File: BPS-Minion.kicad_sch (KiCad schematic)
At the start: 11 parts, among them U12 MIC5317-2.5xM5

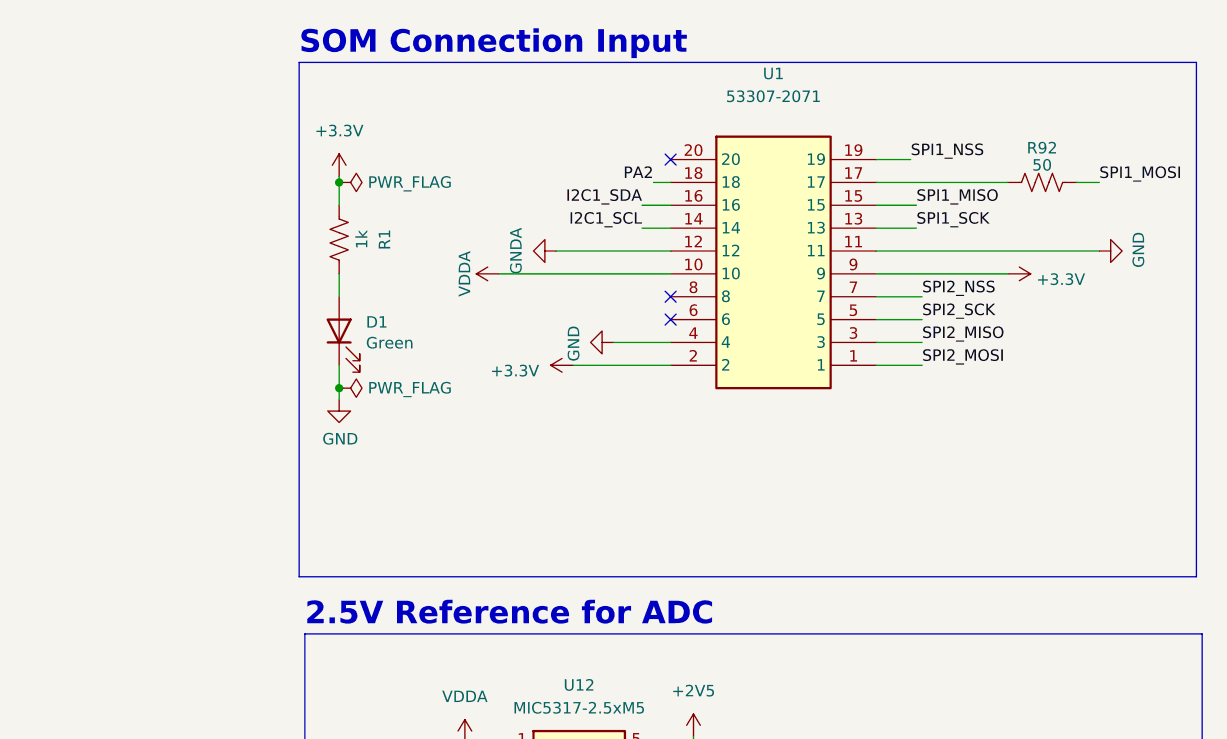
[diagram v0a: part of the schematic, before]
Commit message: wheeeeeee
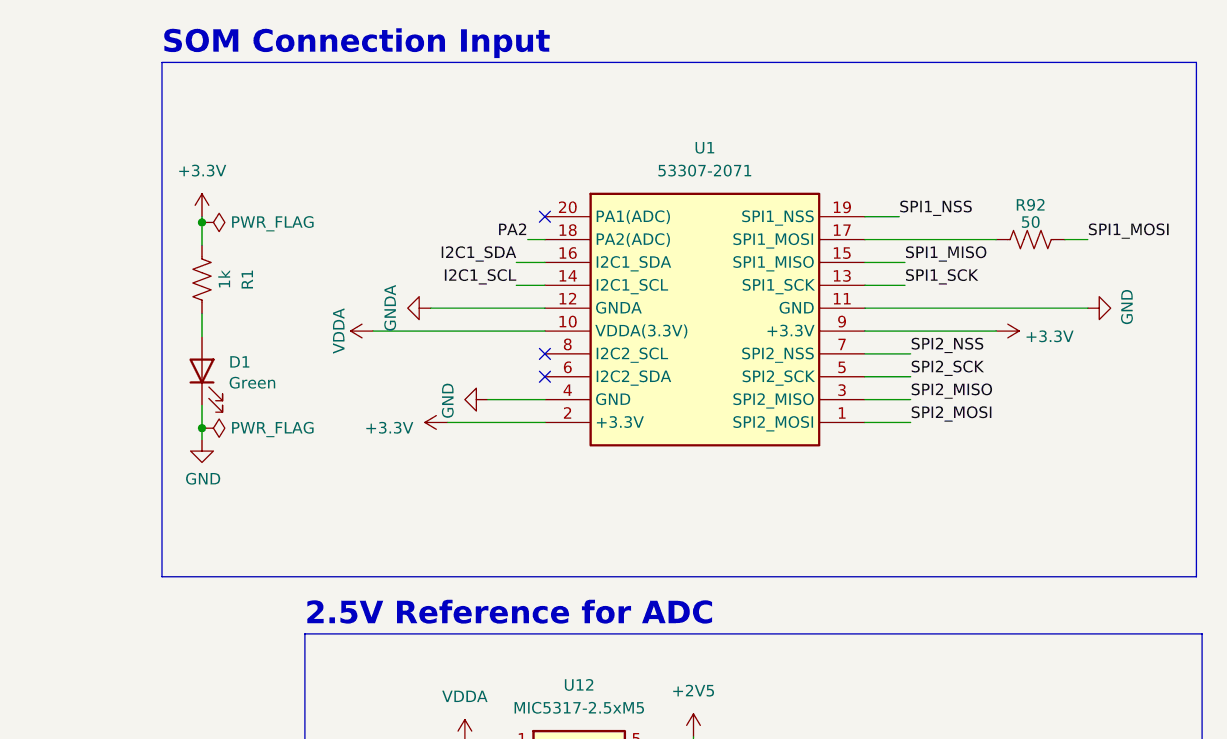
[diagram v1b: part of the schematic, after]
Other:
- moved on the sheet: D1, R1, R92
